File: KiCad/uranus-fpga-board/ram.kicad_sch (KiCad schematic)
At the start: 62 parts, among them U2 NT5CB64M16GP-FL, U3 NT5CB64M16GP-FL, U4 NT5CB64M16GP-FL, U5 NT5CB64M16GP-FL, Y1 SX7DF200.000B20F30DNN

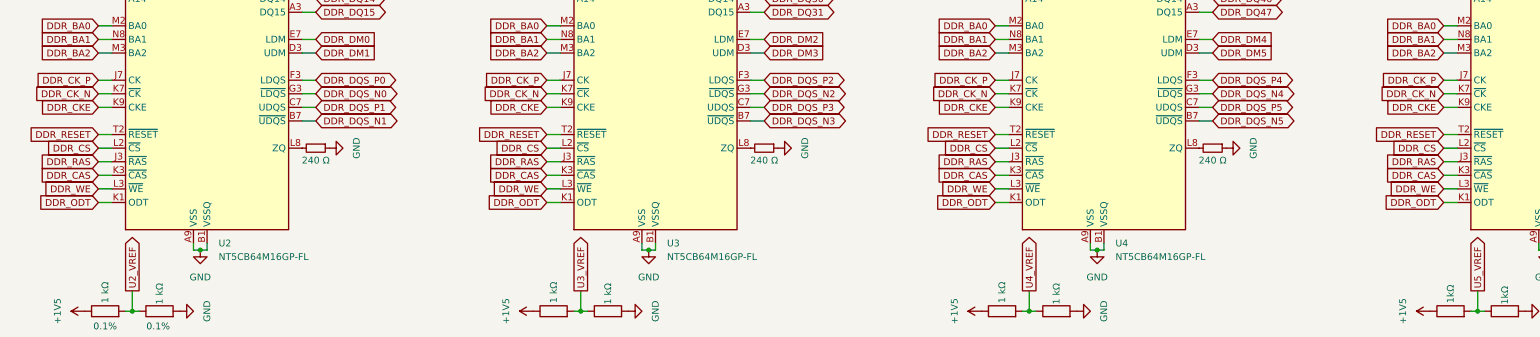
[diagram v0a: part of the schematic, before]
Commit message: Oct 18 journal
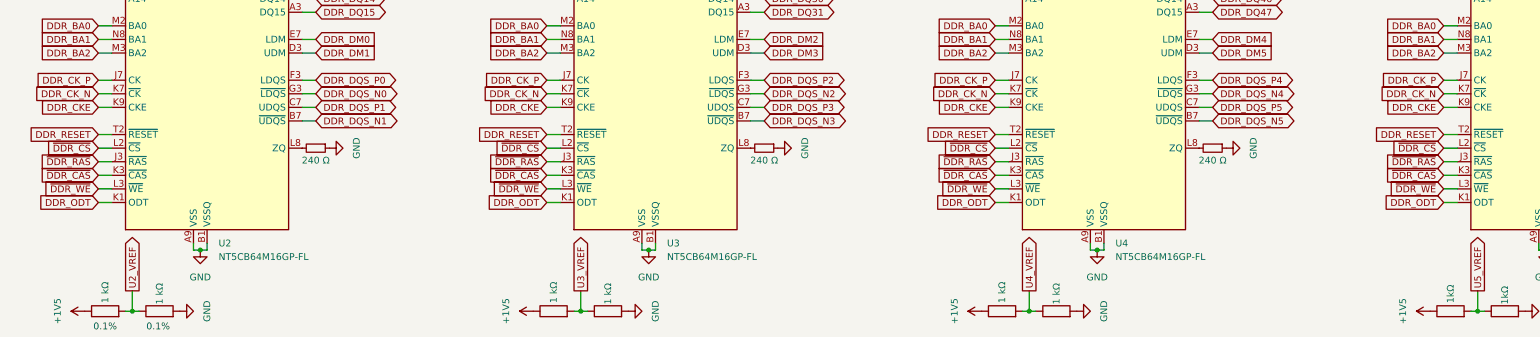
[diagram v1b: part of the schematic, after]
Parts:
- renumbered C44 to C43, C45 to C44, C46 to C45, C47 to C46, C48 to C47, C49 to C48, C50 to C49, C51 to C50, C52 to C51, C43 to C52, C65 to C63, C63 to C64, C64 to C65
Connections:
- net DDR_CAS renamed ~{DDR_CAS}
- net DDR_CS renamed ~{DDR_CS}
- net DDR_RAS renamed ~{DDR_RAS}
- net DDR_WE renamed ~{DDR_WE}
